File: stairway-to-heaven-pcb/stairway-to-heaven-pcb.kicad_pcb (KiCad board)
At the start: 4 copper layers, 99.8 x 97.3 mm, 115 parts, among them J1 Conn_01x04_Male, J10 Conn_01x04_Male, J11 Conn_01x04_Male, J12 Conn_01x04_Male, J13 Conn_01x04_Male, J14 Conn_01x04_Male, J15 PJ-063AH, J16 Conn_01x06_Male, J2 Conn_01x04_Male, J3 Conn_01x04_Male, J4 Conn_01x04_Male, J5 Conn_01x04_Male, J6 Conn_01x04_Male, J7 Conn_01x04_Male, J8 Conn_01x04_Male, J9 Conn_01x04_Male, Q1 FDN337N, Q10 FDN337N, Q11 FDN337N, Q12 FDN337N, Q13 FDN337N, Q14 FDN337N, Q15 FDN337N, Q16 FDN337N, Q17 FDN337N, Q18 FDN337N, Q19 FDN337N, Q2 FDN337N, Q20 FDN337N, Q21 FDN337N, Q22 FDN337N, Q23 FDN337N, Q24 FDN337N, Q25 FDN337N, Q26 FDN337N, Q27 FDN337N, Q28 FDN337N, Q29 FDN337N, Q3 FDN337N, Q30 FDN337N, Q31 FDN337N, Q32 FDN337N, Q33 FDN337N, Q34 FDN337N, Q35 FDN337N, Q36 FDN337N, Q37 FDN337N, Q38 FDN337N, Q39 FDN337N, Q4 FDN337N, Q40 FDN337N, Q41 FDN337N, Q42 FDN337N, Q5 FDN337N, Q6 FDN337N, Q7 FDN337N, Q8 FDN337N, Q9 FDN337N, U1 MEGA_PRO_EMBED_CH340G_{slash}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, U2 LM2575T-5.0

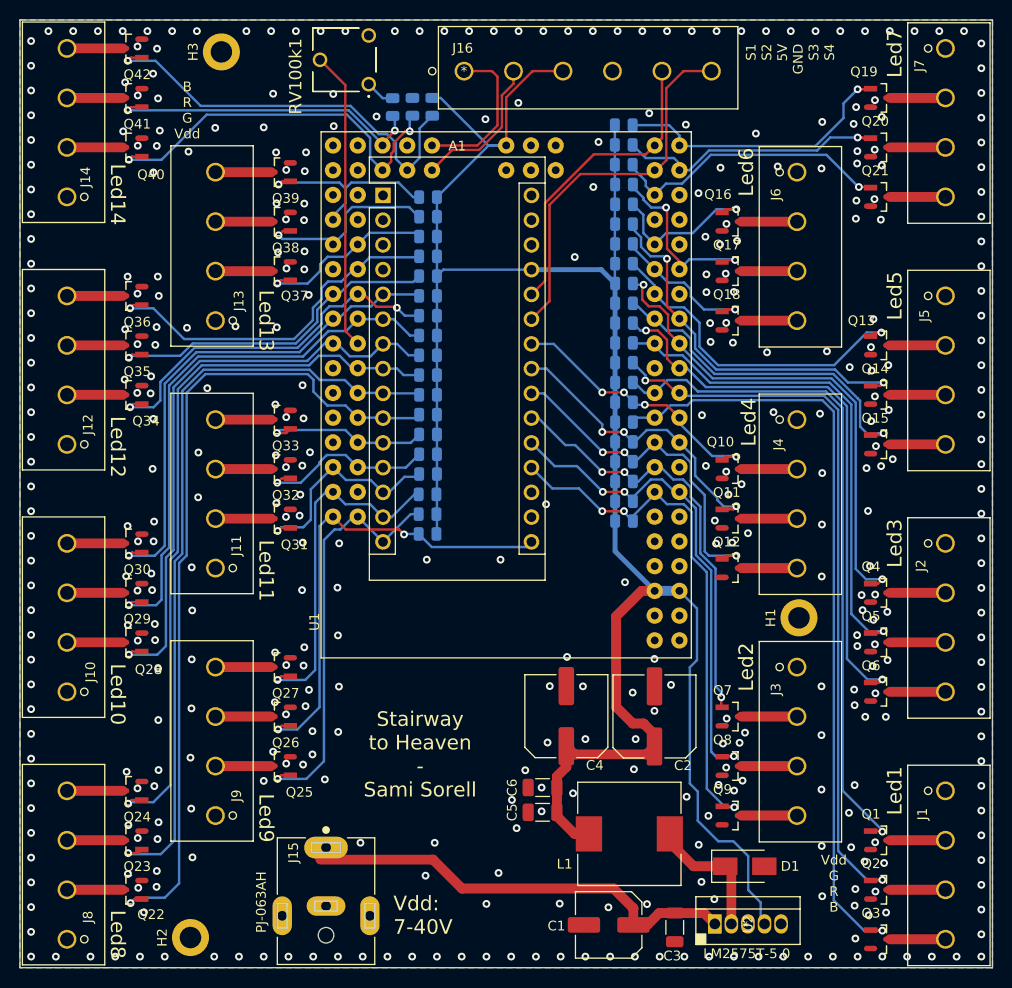
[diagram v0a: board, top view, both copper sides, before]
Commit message: Final touches
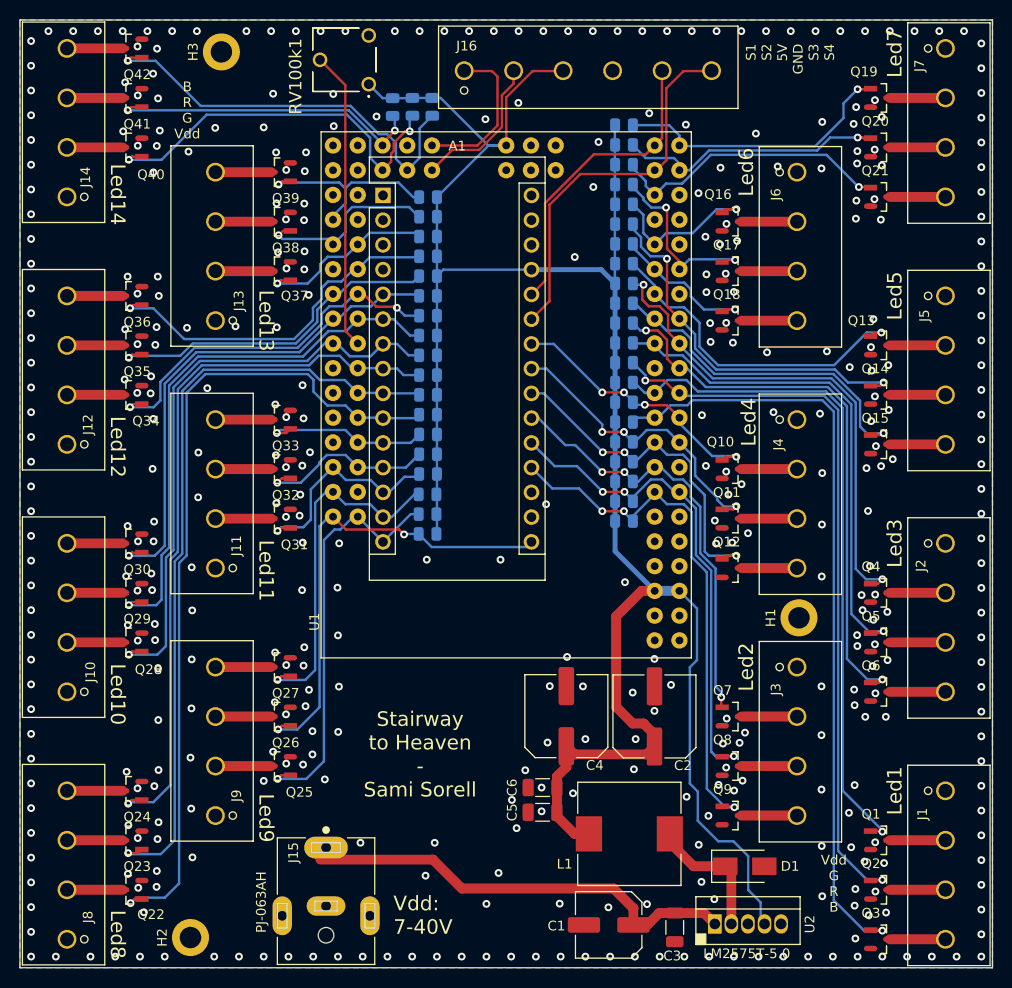
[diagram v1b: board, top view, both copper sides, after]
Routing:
- net +5V: track 221.0 -> 225.0 mm
